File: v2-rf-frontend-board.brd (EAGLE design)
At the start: 160 x 100 mm, 156 parts, among them J1 USB_MICROB, J2 MICROSD, J3 ROCKETNET-CONNECTOR-16M, Q1 NTR4101P, T1 ALT4532, T2 ALT4532, U1 MAX2769, U2 SAW, U3 LAN8710A-EZC, U4 7Q-16.368MBG-T, U5 XC2401, U7 LT4619_REDUCED, U8 STM32F4V, U9 LM3480IM4, X1 25 MHz, X2 BU-SMA-H

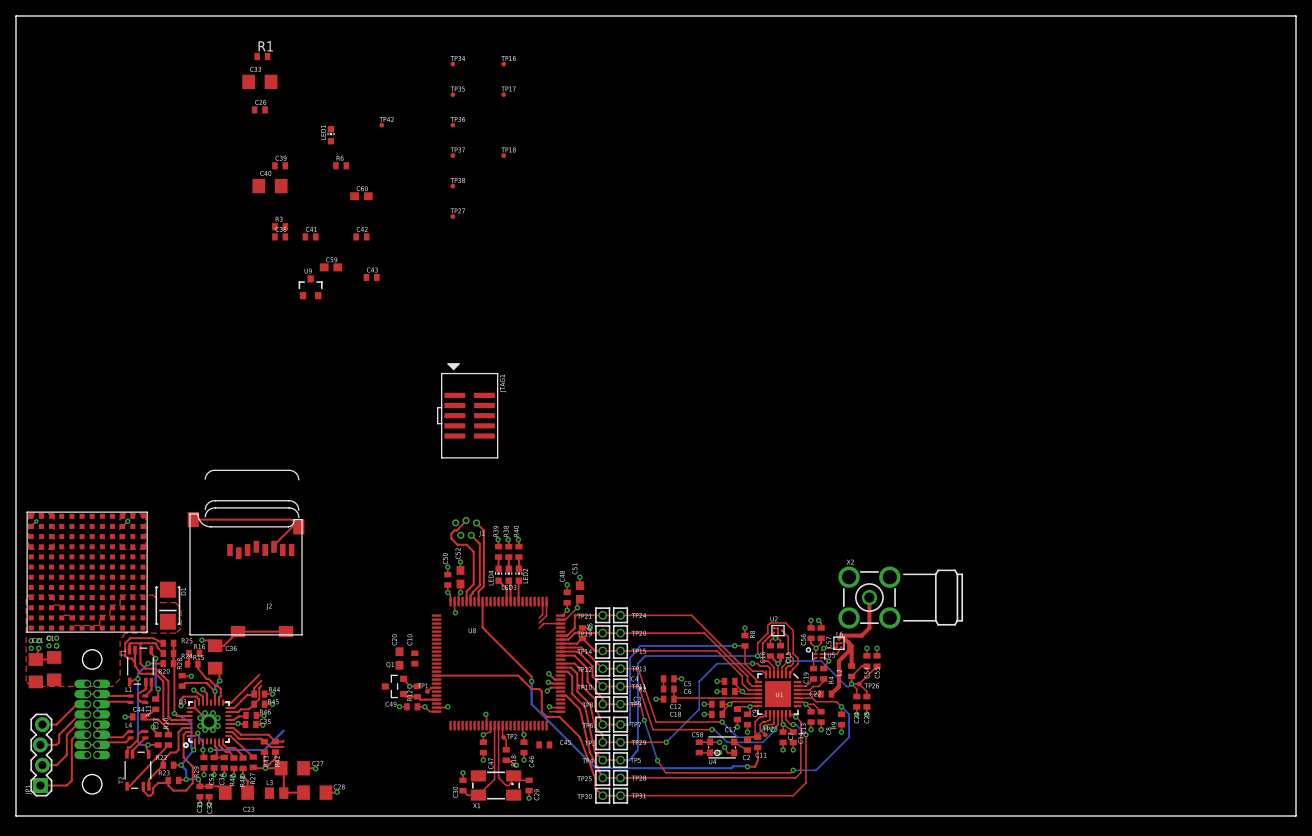
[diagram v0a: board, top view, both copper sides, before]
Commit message: Finished board layout. Removed some test pads. Needs review.
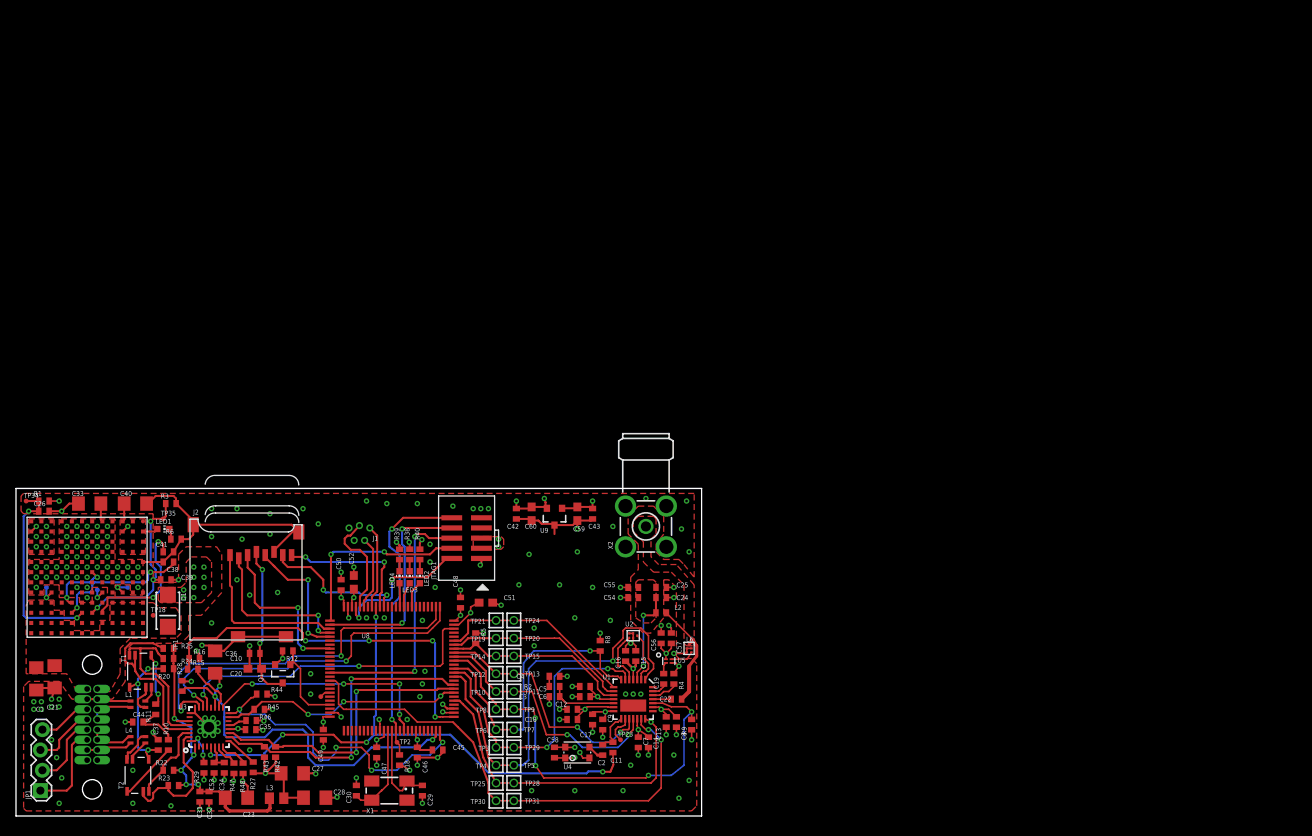
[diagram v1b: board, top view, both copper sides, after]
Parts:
- removed TP26: (no value), testpad:TP06R
- removed TP36, TP37, TP38, TP42: TPTP06R, testpad:TP06R
- TP16, TP17, TP18, TP27, TP34, TP35: value TPTP06R -> (none)
- moved TP17 84.0 mm to (3.81, 28.6), flipped to the bottom
- moved TP16 80.5 mm to (14.0, 28.6), flipped to the bottom
- moved TP34 76.3 mm to (1.27, 39.4)
- moved TP18 72.3 mm to (17.1, 25.1)
- moved TP27 64.5 mm to (10.2, 28.3), flipped to the bottom
- moved TP35 64.2 mm to (18.4, 37.1)
- moved R1 61.9 mm to (3.49, 39.4)
- moved C26 57.0 mm to (3.49, 38.1)
- moved C33 56.8 mm to (9.21, 39.1)
- moved C39 53.7 mm to (18.7, 29.5)
- moved LED1 53.5 mm to (18.4, 35.9), turned to 270 degrees
- moved R6 51.0 mm to (20.0, 34.6), turned to 180 degrees
- moved C60 45.0 mm to (64.5, 37.8), turned to 270 degrees
- moved C59 43.6 mm to (70.2, 37.8), turned to 270 degrees
- moved C41 43.2 mm to (19.1, 33.0)
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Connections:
- net N$17 renamed VFB2
- net +5V: no longer TP37.TP
- net 3.3VA: no longer TP42.TP
- net 3.3VD: no longer TP38.TP
- net ANTBIAS: no longer TP26.TP
- net GND: no longer TP36.TP
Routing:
- net ETH_MDINT: track 2.75 -> 48.4 mm, vias 0 -> 4
- net GND: track 99.8 -> 141.4 mm, vias 61 -> 175
- net ETH_TXD1: track 5.96 -> 47.0 mm, vias 1 -> 2
- net EPHY_NRST: track 9.67 -> 47.6 mm, vias 2 -> 3
- net ETH_TXD0: track 5.22 -> 43.0 mm, vias 1 -> 2
- net ETH_TX_EN: track 4.75 -> 39.6 mm, vias 1 -> 2
- net !RST: track 3.22 -> 37.9 mm, vias 0 -> 2
- net ETH_MDIO: track 5.96 -> 40.4 mm, vias 0 -> 4
- net TDO: track 0.00 -> 32.5 mm, vias 0 -> 2
- net ETH_RXD1: track 9.45 -> 39.4 mm, vias 1 -> 2
- net ETH_RXD0: track 9.18 -> 37.0 mm, vias 1 -> 2
- net TDI: track 0.00 -> 27.4 mm, vias 0 -> 2
- net N$5: track 0.00 -> 25.1 mm, vias 0 -> 2
- net TCK: track 0.00 -> 24.0 mm, vias 0 -> 2
- net ETH_MDC: track 5.98 -> 29.5 mm, vias 0 -> 4
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- added copper zone on layer 2, net +5V
- added copper zone on layer 1, net ANTBIAS
- added copper zone on layer 1, net GND
- added copper zone on layer 1, net LNA2
- added copper zone on layer 1, net OTG_FS_VBUS
- added copper zone on layer 2, net OTG_FS_VBUS
- removed copper zone on layer 2, net VIN
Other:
- board size 160 x 100 mm -> 85.7 x 40.9 mm
